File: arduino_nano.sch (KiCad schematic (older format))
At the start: 1 part

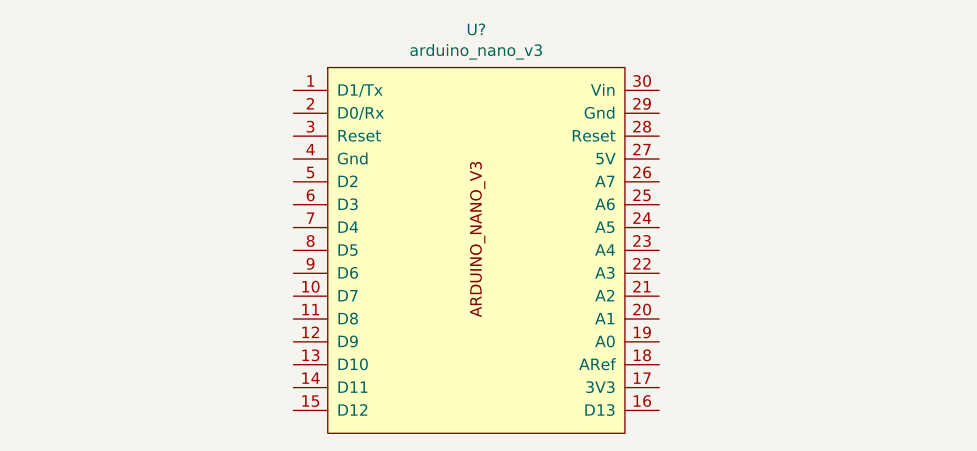
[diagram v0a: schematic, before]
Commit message: update,
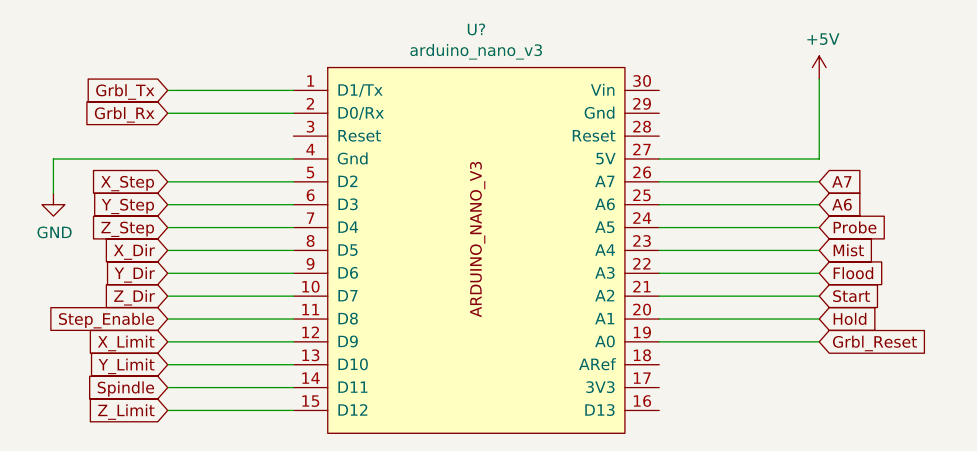
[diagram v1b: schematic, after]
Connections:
- net Grbl_Tx: now reaches U?.1 (D1/Tx)
- net Z_Dir: now reaches U?.10 (D7)
- net Step_Enable: now reaches U?.11 (D8)
- net X_Limit: now reaches U?.12 (D9)
- net Y_Limit: now reaches U?.13 (D10)
- net Spindle: now reaches U?.14 (D11)
- net Z_Limit: now reaches U?.15 (D12)
- net Grbl_Reset: now reaches U?.19 (A0)
- net Grbl_Rx: now reaches U?.2 (D0/Rx)
- net Hold: now reaches U?.20 (A1)
- net Start: now reaches U?.21 (A2)
- net Flood: now reaches U?.22 (A3)
- net Mist: now reaches U?.23 (A4)
- net Probe: now reaches U?.24 (A5)
- net A6: now reaches U?.25 (A6)
- net A7: now reaches U?.26 (A7)
- net +5V: now reaches U?.27 (5V)
- net GND: now reaches U?.4 (Gnd)
- net X_Step: now reaches U?.5 (D2)
- net Y_Step: now reaches U?.6 (D3)
- net Z_Step: now reaches U?.7 (D4)
- net X_Dir: now reaches U?.8 (D5)
- net Y_Dir: now reaches U?.9 (D6)
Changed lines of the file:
@@
 	1    0    0    -1
 $EndComp
+Text GLabel 4500 2950 0    50   Input ~ 0
+Grbl_Tx
+Text GLabel 4500 3050 0    50   Input ~ 0
+Grbl_Rx
+Text GLabel 4500 3350 0    50   Input ~ 0
+X_Step
+Text GLabel 4500 3450 0    50   Input ~ 0
+Y_Step
+Text GLabel 4500 3550 0    50   Input ~ 0
+Z_Step
+Text GLabel 4500 3650 0    50   Input ~ 0
+X_Dir
+Text GLabel 4500 3750 0    50   Input ~ 0
+Y_Dir
+Text GLabel 4500 3850 0    50   Input ~ 0
+Z_Dir
+Text GLabel 4500 3950 0    50   Input ~ 0
+Step_Enable
+Text GLabel 4500 4050 0    50   Input ~ 0
+X_Limit
+Text GLabel 4500 4150 0    50   Input ~ 0
+Y_Limit
+Text GLabel 4500 4250 0    50   Input ~ 0
+Spindle
+Text GLabel 4500 4350 0    50   Input ~ 0
+Z_Limit
+Wire Wire Line
+	4500 2950 5050 2950
+Wire Wire Line
+	4500 3050 5050 3050
+Wire Wire Line
+	4500 3350 5050 3350
+Wire Wire Line
+	4500 3450 5050 3450
+Wire Wire Line
+	4500 3550 5050 3550
+Wire Wire Line
+	4500 3650 5050 3650
+Wire Wire Line
+	4500 3750 5050 3750
+Wire Wire Line
+	4500 3850 5050 3850
+Wire Wire Line
+	4500 3950 5050 3950
+Wire Wire Line
+	4500 4050 5050 4050
+Wire Wire Line
+	4500 4150 5050 4150
+Wire Wire Line
+	4500 4250 5050 4250
+Wire Wire Line
+	4500 4350 5050 4350
+$Comp
+L power:GND #PWR?
+U 1 1 5BFF107B
+P 4000 3400
+F 0 "#PWR?" H 4000 3150 50  0001 C CNN
+F 1 "GND" H 4005 3227 50  0000 C CNN
+F 2 "" H 4000 3400 50  0001 C CNN
+F 3 "" H 4000 3400 50  0001 C CNN
+	1    4000 3400
+	1    0    0    -1
+$EndComp
+Wire Wire Line
+	4000 3400 4000 3250
+Wire Wire Line
+	4000 3250 5050 3250
+Text GLabel 7350 3350 2    50   Input ~ 0
+A7
+Text GLabel 7350 3450 2    50   Input ~ 0
+A6
+Text GLabel 7350 3550 2    50   Input ~ 0
+Probe
+Text GLabel 7350 3650 2    50   Input ~ 0
+Mist
+Text GLabel 7350 3750 2    50   Input ~ 0
+Flood
+Text GLabel 7350 3850 2    50   Input ~ 0
+Start
+Text GLabel 7350 3950 2    50   Input ~ 0
+Hold
+Text GLabel 7350 4050 2    50   Input ~ 0
+Grbl_Reset
+$Comp
+L tinkerforge:+5V #PWR?
+U 1 1 5BFF1342
+P 7350 2900
+F 0 "#PWR?" H 7350 2750 50  0001 C CNN
+F 1 "+5V" H 7365 3073 50  0000 C CNN
+F 2 "" H 7350 2900 50  0000 C CNN
+F 3 "" H 7350 2900 50  0000 C CNN
+	1    7350 2900
+	1    0    0    -1
+$EndComp
+Wire Wire Line
+	6650 3250 7350 3250
+Wire Wire Line
+	7350 3250 7350 2900
+Wire Wire Line
+	6650 3350 7350 3350
+Wire Wire Line
+	6650 3450 7350 3450
+Wire Wire Line
+	6650 3550 7350 3550
+Wire Wire Line
+	6650 3650 7350 3650
+Wire Wire Line
+	6650 3750 7350 3750
+Wire Wire Line
+	6650 3850 7350 3850
+Wire Wire Line
+	6650 3950 7350 3950
+Wire Wire Line
+	6650 4050 7350 4050
 $EndSCHEMATC
